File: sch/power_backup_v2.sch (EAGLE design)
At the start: 38 parts, among them IC1 78L05SMD, IC2 ACS712-LC, K1 DS2Y-S-DC48V, T1 BC847, T2 BC847, T3 BC847, T4 BC847

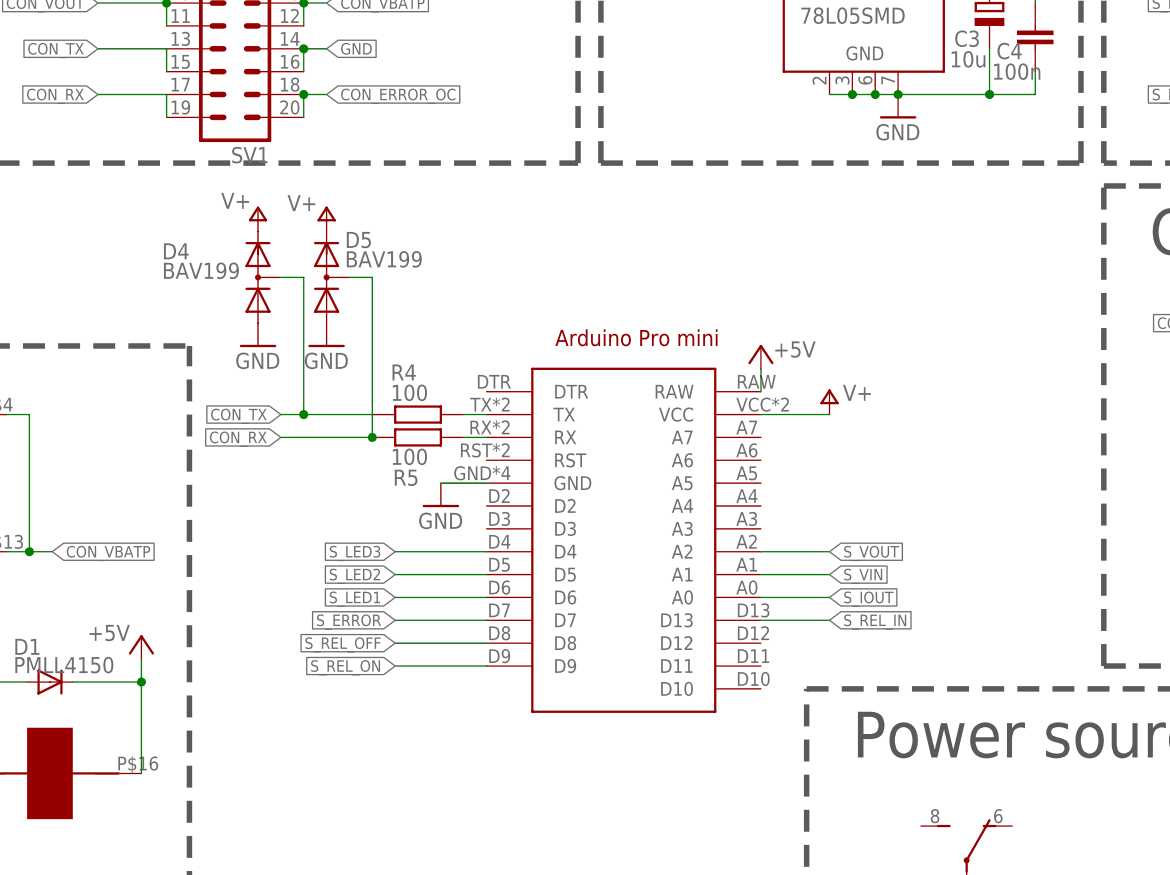
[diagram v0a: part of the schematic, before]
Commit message: updated images
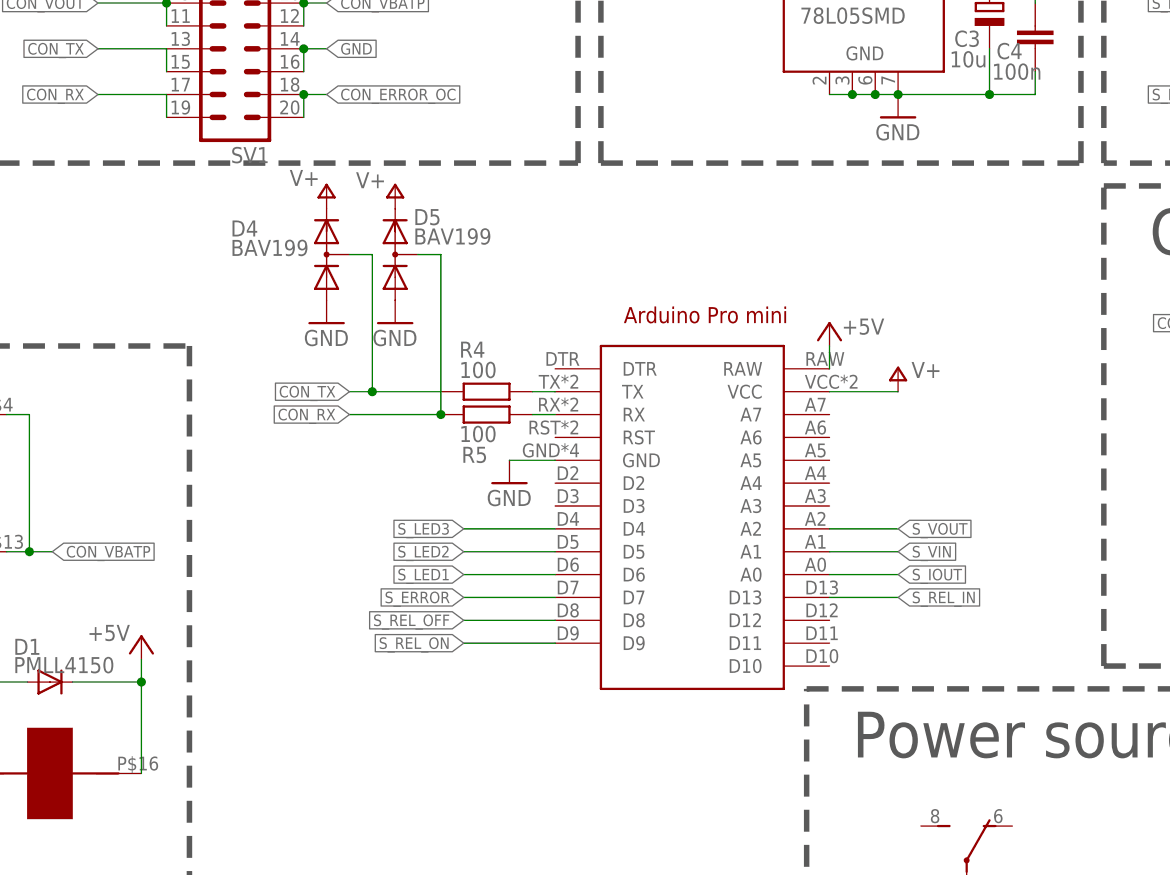
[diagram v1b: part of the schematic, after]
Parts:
- renumbered U$1 to K2
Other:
- moved on the sheet: D4, D5, R4, R5
